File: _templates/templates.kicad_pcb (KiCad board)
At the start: 2 copper layers, 180.2 x 128.5 mm, 0 parts

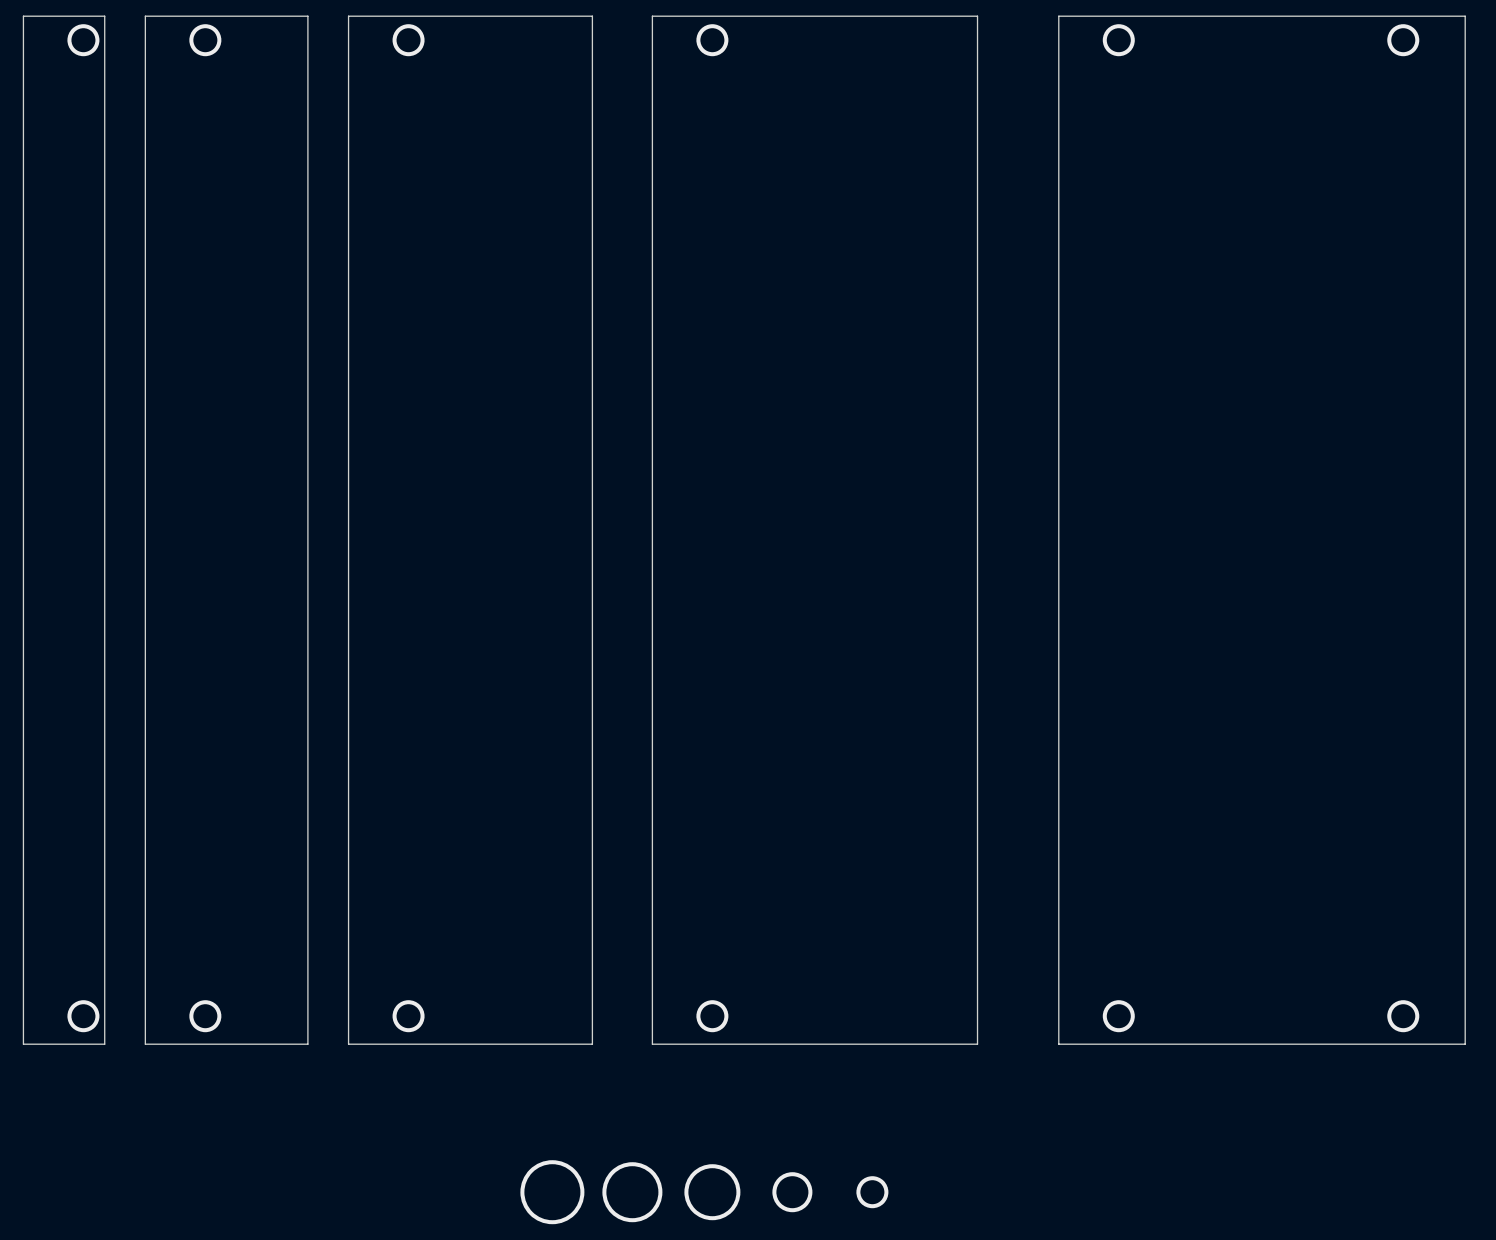
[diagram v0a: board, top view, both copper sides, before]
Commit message: added some 3d models and backlog
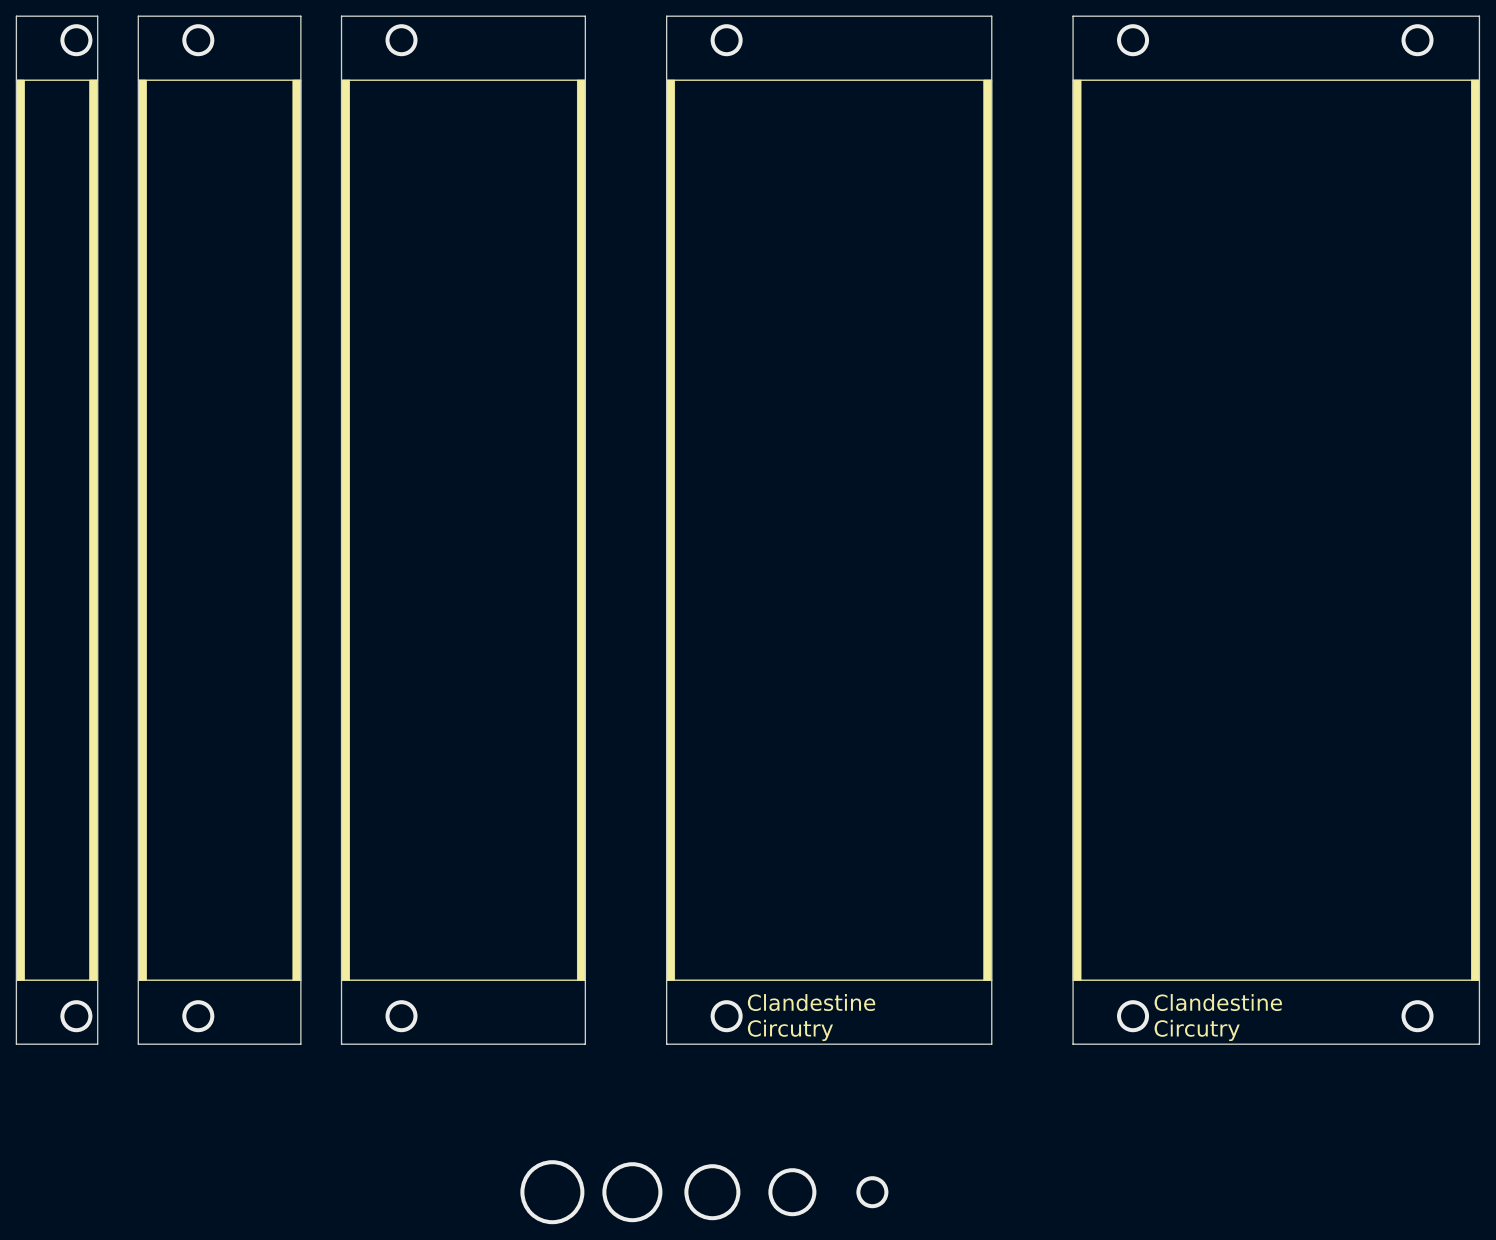
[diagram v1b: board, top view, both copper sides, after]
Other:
- board size 180.2 x 128.5 mm -> 182.9 x 128.5 mm
- board text added: "Clandestine Circutry"
